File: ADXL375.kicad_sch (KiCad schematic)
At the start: 5 parts, among them U12 ADXL375BCCZ

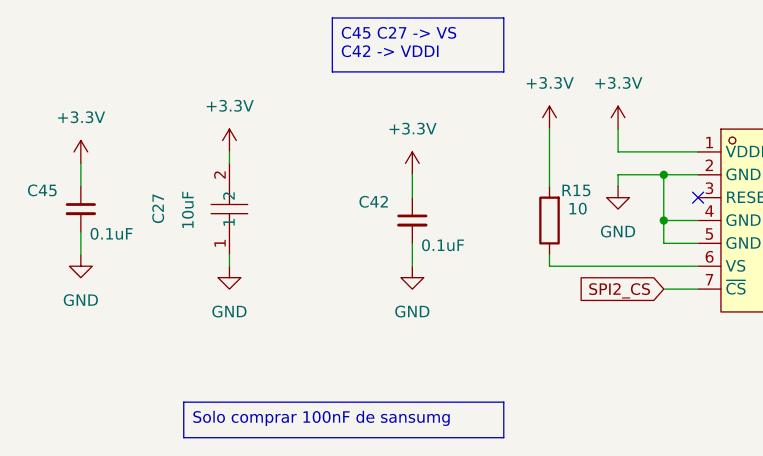
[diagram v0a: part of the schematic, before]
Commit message: jhamir
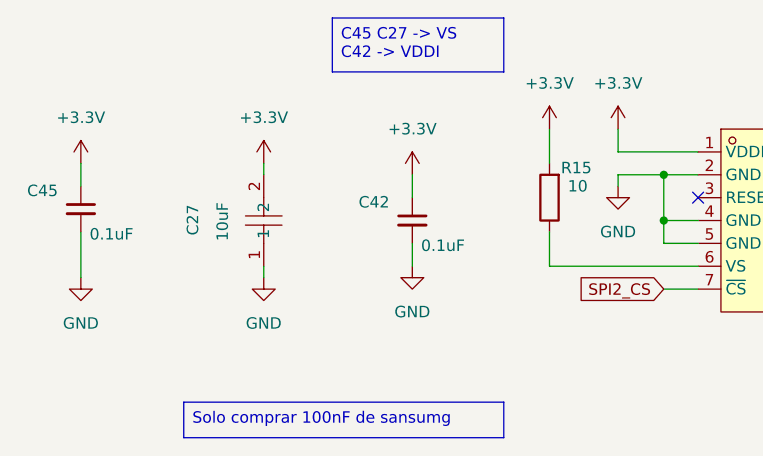
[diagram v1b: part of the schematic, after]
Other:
- moved on the sheet: C27, R15
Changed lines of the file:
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@@
 	(wire
 		(pts
-			(xy 49.53 93.98) (xy 49.53 95.25)
+			(xy 53.34 95.25) (xy 53.34 96.52)
 		)
 		(stroke
@@
 	(wire
 		(pts
-			(xy 85.09 80.01) (xy 85.09 86.36)
+			(xy 85.09 80.01) (xy 85.09 83.82)
 		)
 		(stroke
@@
 	(wire
 		(pts
-			(xy 33.02 91.44) (xy 33.02 93.98)
+			(xy 33.02 91.44) (xy 33.02 96.52)
 		)
 		(stroke
@@
 	(wire
 		(pts
-			(xy 85.09 93.98) (xy 85.09 95.25)
+			(xy 85.09 91.44) (xy 85.09 95.25)
 		)
 		(stroke
@@
 	(wire
 		(pts
-			(xy 49.53 82.55) (xy 49.53 83.82)
+			(xy 53.34 83.82) (xy 53.34 85.09)
 		)
 		(stroke
@@
 	(symbol
 		(lib_id "power:GND")
-		(at 33.02 93.98 0)
+		(at 33.02 96.52 0)
 		(mirror y)
 		(unit 1)
@@
 		(fields_autoplaced yes)
 		(property "Reference" "#PWR0136"
-			(at 33.02 100.33 0)
+			(at 33.02 102.87 0)
 			(hide yes)
 			(show_name no)
@@
 		)
 		(property "Value" "GND"
-			(at 33.02 99.06 0)
+			(at 33.02 101.6 0)
 			(show_name no)
 			(do_not_autoplace no)
@@
 		)
 		(property "Footprint" ""
-			(at 33.02 93.98 0)
+			(at 33.02 96.52 0)
 			(hide yes)
 			(show_name no)
@@
 		)
 		(property "Datasheet" ""
-			(at 33.02 93.98 0)
+			(at 33.02 96.52 0)
 			(hide yes)
 			(show_name no)
@@
 		)
 		(property "Description" "Power symbol creates a global label with name \"GND\" , ground"
-			(at 33.02 93.98 0)
+			(at 33.02 96.52 0)
 			(hide yes)
 			(show_name no)
@@
 	(symbol
 		(lib_id "power:+3.3V")
-		(at 49.53 82.55 0)
+		(at 53.34 83.82 0)
 		(unit 1)
 		(body_style 1)
@@
 		(fields_autoplaced yes)
 		(property "Reference" "#PWR0131"
-			(at 49.53 86.36 0)
+			(at 53.34 87.63 0)
 			(hide yes)
 			(show_name no)
@@
 		)
 		(property "Value" "+3.3V"
-			(at 49.53 77.47 0)
+			(at 53.34 78.74 0)
 			(show_name no)
 			(do_not_autoplace no)
@@
 		)
 		(property "Footprint" ""
-			(at 49.53 82.55 0)
+			(at 53.34 83.82 0)
 			(hide yes)
 			(show_name no)
@@
 		)
 		(property "Datasheet" ""
-			(at 49.53 82.55 0)
+			(at 53.34 83.82 0)
 			(hide yes)
 			(show_name no)
@@
 		)
 		(property "Description" "Power symbol creates a global label with name \"+3.3V\""
-			(at 49.53 82.55 0)
+			(at 53.34 83.82 0)
 			(hide yes)
 			(show_name no)
@@
 	(symbol
 		(lib_id "power:GND")
-		(at 49.53 95.25 0)
+		(at 53.34 96.52 0)
 		(mirror y)
 		(unit 1)
@@
 		(fields_autoplaced yes)
 		(property "Reference" "#PWR0132"
-			(at 49.53 101.6 0)
+			(at 53.34 102.87 0)
 			(hide yes)
 			(show_name no)
@@
 		)
 		(property "Value" "GND"
-			(at 49.53 100.33 0)
+			(at 53.34 101.6 0)
 			(show_name no)
 			(do_not_autoplace no)
@@
 		)
 		(property "Footprint" ""
-			(at 49.53 95.25 0)
+			(at 53.34 96.52 0)
 			(hide yes)
 			(show_name no)
@@
 		)
 		(property "Datasheet" ""
-			(at 49.53 95.25 0)
+			(at 53.34 96.52 0)
 			(hide yes)
 			(show_name no)
@@
 		)
 		(property "Description" "Power symbol creates a global label with name \"GND\" , ground"
-			(at 49.53 95.25 0)
+			(at 53.34 96.52 0)
 			(hide yes)
 			(show_name no)
@@
 	(symbol
 		(lib_id "Device:R")
-		(at 85.09 90.17 180)
+		(at 85.09 87.63 180)
 		(unit 1)
 		(body_style 1)
@@
 		(dnp no)
 		(property "Reference" "R15"
-			(at 86.36 86.868 0)
+			(at 86.36 84.328 0)
 			(show_name no)
 			(do_not_autoplace no)
@@
 		)
 		(property "Value" "10"
-			(at 87.122 88.9 0)
+			(at 87.122 86.36 0)
 			(show_name no)
 			(do_not_autoplace no)
@@
 		)
 		(property "Footprint" "Resistor_SMD:R_0603_1608Metric_Pad0.98x0.95mm_HandSolder"
-			(at 86.868 90.17 90)
+			(at 86.868 87.63 90)
 			(hide yes)
 			(show_name no)
@@
 		)
 		(property "Datasheet" "C163851"
-			(at 85.09 90.17 0)
+			(at 85.09 87.63 0)
 			(hide yes)
 			(show_name no)
@@
 		)
 		(property "Description" "Resistor"
-			(at 85.09 90.17 0)
+			(at 85.09 87.63 0)
 			(hide yes)
 			(show_name no)
@@
 		)
 		(property "Field7" ""
-			(at 85.09 90.17 90)
+			(at 85.09 87.63 90)
 			(hide yes)
 			(show_name no)
@@
 	(symbol
 		(lib_id "CANSAT_STM32_symbols:CL21B106KAYQNNE")
-		(at 49.53 88.9 90)
+		(at 53.34 90.17 90)
 		(unit 1)
 		(body_style 1)
@@
 		(dnp no)
 		(property "Reference" "C27"
-			(at 41.656 87.122 0)
+			(at 45.466 88.392 0)
 			(show_name no)
 			(do_not_autoplace no)
@@
 		)
 		(property "Value" "10uF"
-			(at 44.958 86.868 0)
+			(at 48.768 88.138 0)
 			(show_name no)
 			(do_not_autoplace no)
@@
 		)
 		(property "Footprint" "Capacitor_SMD:C_0805_2012Metric_Pad1.18x1.45mm_HandSolder"
-			(at 57.15 88.9 0)
+			(at 60.96 90.17 0)
 			(hide yes)
 			(show_name no)
@@
 		)
 		(property "Datasheet" "https://www.lcsc.com/datasheet/C3039694.pdf"
-			(at 59.69 88.9 0)
+			(at 63.5 90.17 0)
 			(hide yes)
 			(show_name no)
@@
 		)
 		(property "Description" ""
-			(at 49.53 88.9 0)
+			(at 53.34 90.17 0)
 			(hide yes)
 			(show_name no)
@@
 		)
 		(property "Manufacturer" "SAMSUNG(三星)"
-			(at 62.23 88.9 0)
+			(at 66.04 90.17 0)
 			(hide yes)
 			(show_name no)
@@
 		)
 		(property "MPN" "CL21B106KAYQNNE"
-			(at 64.77 88.9 0)
+			(at 68.58 90.17 0)
 			(hide yes)
 			(show_name no)
@@
 		)
 		(property "LCSC Part" "C3039694"
-			(at 67.31 88.9 0)
+			(at 71.12 90.17 0)
 			(hide yes)
 			(show_name no)

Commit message: PLACA FINISHED
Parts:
- C42, C45: Link https://www.lcsc.com/product-detail/C1590.html -> (none)
- U12: Link https://www.lcsc.com/product-detail/C481898.html -> (none)
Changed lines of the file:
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@@
-			)
-		)
-		(property "Link" "https://www.lcsc.com/product-detail/C481898.html"
-			(at 124.46 90.17 0)
-			(hide yes)
-			(show_name no)
-			(do_not_autoplace no)
-			(effects
-				(font
-					(size 1.27 1.27)
-				)
 			)
 		)
@@
 			)
 		)
-		(property "Link" "https://www.lcsc.com/product-detail/C1590.html"
-			(at 33.02 88.9 0)
-			(hide yes)
-			(show_name no)
-			(do_not_autoplace no)
-			(effects
-				(font
-					(size 1.27 1.27)
-				)
-			)
-		)
 		(pin "1"
 		)
@@
 			(at 69.85 90.17 0)
 			(hide yes)
-			(show_name no)
-			(do_not_autoplace no)
-			(effects
-				(font
-					(size 1.27 1.27)
-				)
-			)
-		)
-		(property "Link" "https://www.lcsc.com/product-detail/C1590.html"
-			(at 69.85 90.17 0)
-			(hide yes)
